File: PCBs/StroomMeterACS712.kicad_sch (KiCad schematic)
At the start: 22 parts, among them J1 OLED1604, J2 ACS712, J3 PWR_5V_pin, J4 WS2812, J5 PWR_5V_jst, J6 Voeding_in, K1 SRD-03VDC-SL-C, Q1 BC547, Q2 BC547, SW1 btnAanUit, SW2 SW_SPDT, U1 WeMos_D1_mini, U2 PCF8574A

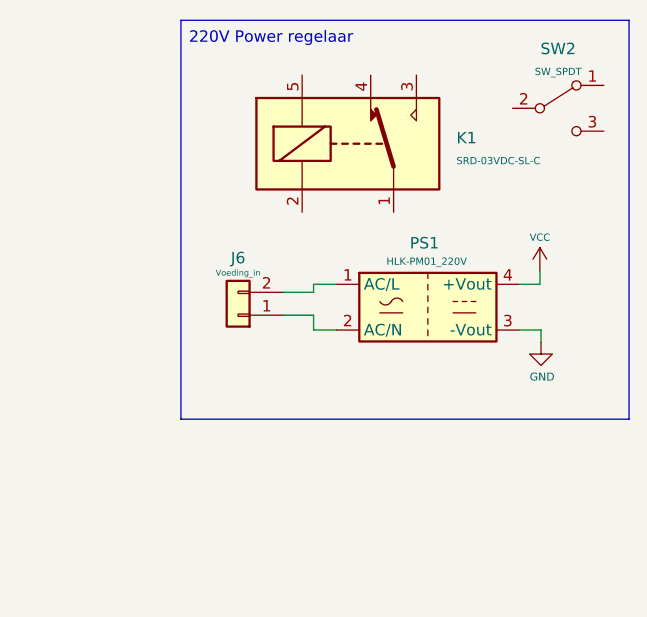
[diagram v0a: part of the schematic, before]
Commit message: Bijgewerkt
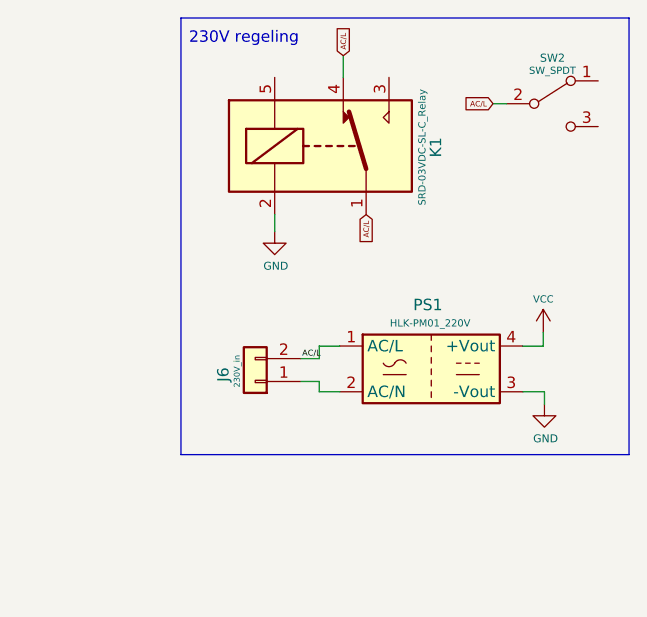
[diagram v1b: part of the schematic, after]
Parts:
- J6: value Voeding_in -> 230V_in
- K1: value SRD-03VDC-SL-C -> SRD-03VDC-SL-C_Relay
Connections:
- net GND: now also K1.2
- net AC/L: now reaches J6.2 (Pin_2), PS1.1 (AC/L)
- net AC/L: now also K1.1, K1.4, SW2.2 (B)
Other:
- note added: "230V regeling"
- note removed: "220V Power regelaar"
- moved on the sheet: J6, K1, PS1, SW2
